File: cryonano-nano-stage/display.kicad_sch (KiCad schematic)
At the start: 1 part, among them U3 1ED3141MU12FXUMA1

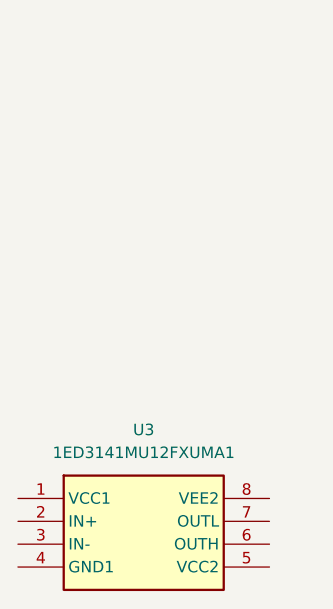
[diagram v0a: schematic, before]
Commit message: preliminary components added
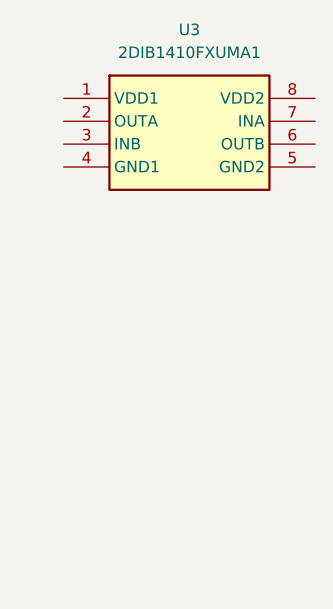
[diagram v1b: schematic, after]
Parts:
- removed U3: 1ED3141MU12FXUMA1, SOIC127P600X175-8N, symbol symbols:1ED3141MU12FXUMA1
- added U3: 2DIB1410FXUMA1, SOIC127P600X175-8N, symbol symbols:2DIB1410FXUMA1
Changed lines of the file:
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@@
 	(paper "A4")
 	(symbol
-		(lib_id "symbols:1ED3141MU12FXUMA1")
-		(at 101.6 101.6 0)
+		(lib_id "symbols:2DIB1410FXUMA1")
+		(at 106.68 57.15 0)
 		(unit 1)
 		(body_style 1)
@@
 		(fields_autoplaced yes)
 		(property "Reference" "U3"
-			(at 115.57 93.98 0)
+			(at 120.65 49.53 0)
 			(show_name no)
 			(do_not_autoplace no)
@@
 			)
 		)
-		(property "Value" "1ED3141MU12FXUMA1"
-			(at 115.57 96.52 0)
+		(property "Value" "2DIB1410FXUMA1"
+			(at 120.65 52.07 0)
 			(show_name no)
 			(do_not_autoplace no)
@@
 		)
 		(property "Footprint" "SOIC127P600X175-8N"
-			(at 125.73 196.52 0)
+			(at 130.81 152.07 0)
 			(hide yes)
 			(show_name no)
@@
 			)
 		)
-		(property "Datasheet" "https://www.mouser.in/datasheet/2/196/Infineon_1ED314xMU12F_DataSheet_v01_00_EN-3106223.pdf"
-			(at 125.73 296.52 0)
+		(property "Datasheet" "https://www.infineon.com/dgdl/Infineon-2DIBx41xF-DS_v01_00-EN.pdf-DataSheet-v01_00-EN.pdf?fileId=8ac78c8c872bd8d60187370abe7d246c"
+			(at 130.81 252.07 0)
 			(hide yes)
 			(show_name no)
@@
 			)
 		)
-		(property "Description" "Galvanically Isolated Gate Drivers ISOLATED DRIVER"
-			(at 101.6 101.6 0)
+		(property "Description" "General Purpose Digital Isolator 3000Vrms 2 Channel 40Mbps 100kV/s CMTI 8-SOIC (0.154\", 3.90mm Width)"
+			(at 106.68 57.15 0)
 			(hide yes)
 			(show_name no)
@@
 		)
 		(property "Height" "1.75"
-			(at 125.73 496.52 0)
+			(at 130.81 452.07 0)
 			(hide yes)
 			(show_name no)
@@
 		)
 		(property "element14 Part Number" ""
-			(at 125.73 596.52 0)
+			(at 130.81 552.07 0)
 			(hide yes)
 			(show_name no)
@@
 		)
 		(property "element14 Price/Stock" ""
-			(at 125.73 696.52 0)
+			(at 130.81 652.07 0)
 			(hide yes)
 			(show_name no)
@@
 		)
 		(property "Manufacturer_Name" "Infineon"
-			(at 125.73 796.52 0)
+			(at 130.81 752.07 0)
 			(hide yes)
 			(show_name no)
@@
 			)
 		)
-		(property "Manufacturer_Part_Number" "1ED3141MU12FXUMA1"
-			(at 125.73 896.52 0)
+		(property "Manufacturer_Part_Number" "2DIB1410FXUMA1"
+			(at 130.81 852.07 0)
 			(hide yes)
 			(show_name no)
@@
 			)
 		)
-		(pin "6"
-		)
 		(pin "5"
-		)
-		(pin "7"
-		)
-		(pin "1"
 		)
 		(pin "2"
 		)
-		(pin "3"
+		(pin "7"
 		)
 		(pin "4"
@@
 		(pin "8"
 		)
+		(pin "1"
+		)
+		(pin "3"
+		)
+		(pin "6"
+		)
 		(instances
 			(project "cryonano-nano-stage"
-				(path "/549c6da5-71cb-4d9c-a0a2-c409a6f93509/37ffb213-c706-4fdf-aede-61f2739d8503/134546d9-2553-4cbc-b149-ff74fa29d06b"
+				(path "/549c6da5-71cb-4d9c-a0a2-c409a6f93509/ad264f78-6ca8-4bc7-89c7-bd7bbd97c564"
 					(reference "U3")
 					(unit 1)
